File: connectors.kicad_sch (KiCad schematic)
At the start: 4 parts, among them J1 Conn_01x04_Pin, J2 Conn_01x04_Pin, J3 Conn_01x09_Pin, J4 Conn_02x03_Odd_Even

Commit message: Completed symbol-footprint associations
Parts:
- J1, J2: footprint (none) -> Connector_PinHeader_2.54mm:PinHeader_1x04_P2.54mm_Vertical
- J3: footprint (none) -> Connector_PinHeader_2.54mm:PinHeader_1x09_P2.54mm_Vertical
- J4: footprint (none) -> Connector_PinHeader_2.54mm:PinHeader_2x03_P2.54mm_Vertical
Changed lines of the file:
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@@
 			)
 		)
-		(property "Footprint" ""
+		(property "Footprint" "Connector_PinHeader_2.54mm:PinHeader_1x04_P2.54mm_Vertical"
 			(at 82.55 66.04 0)
 			(hide yes)
@@
 			)
 		)
-		(property "Footprint" ""
+		(property "Footprint" "Connector_PinHeader_2.54mm:PinHeader_1x04_P2.54mm_Vertical"
 			(at 60.96 66.04 0)
 			(hide yes)
@@
 			)
 		)
-		(property "Footprint" ""
+		(property "Footprint" "Connector_PinHeader_2.54mm:PinHeader_1x09_P2.54mm_Vertical"
 			(at 60.96 96.52 0)
 			(hide yes)
@@
 			)
 		)
-		(property "Footprint" ""
+		(property "Footprint" "Connector_PinHeader_2.54mm:PinHeader_2x03_P2.54mm_Vertical"
 			(at 83.82 90.17 0)
 			(hide yes)

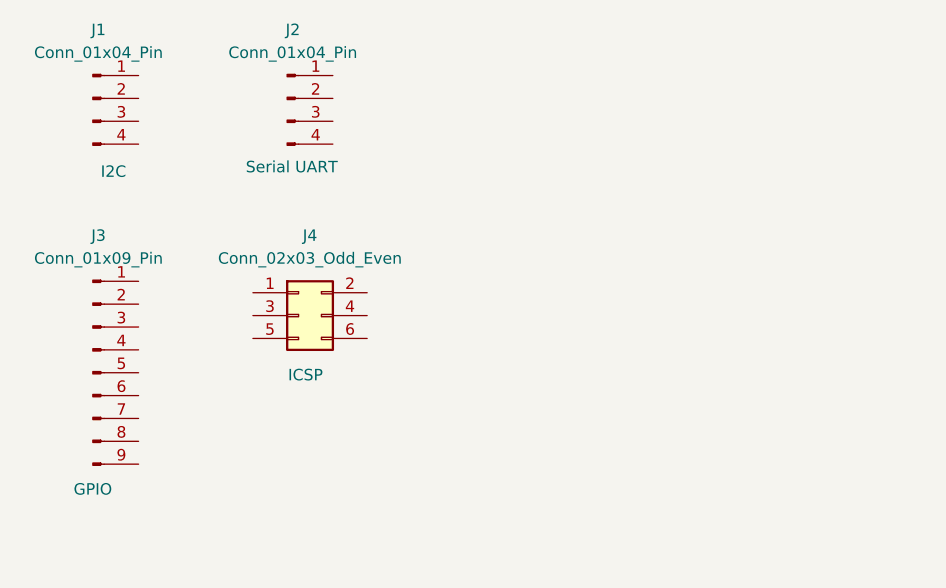
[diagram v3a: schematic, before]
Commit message: Completed wiring of the second sheet
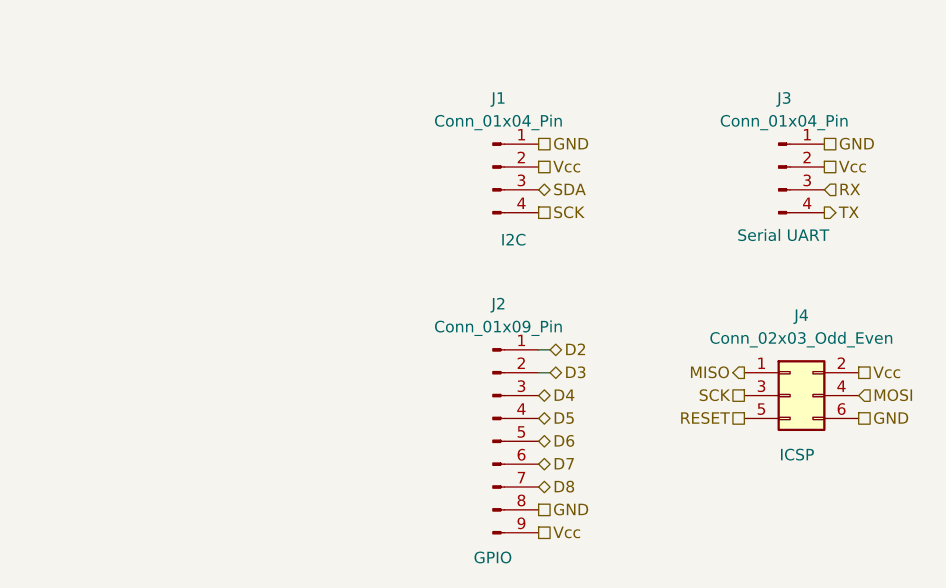
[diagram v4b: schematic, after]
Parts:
- renumbered J3 to J2, J2 to J3
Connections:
- net GND: now reaches J3.1 (Pin_1)
- net GND: now also J1.1 (Pin_1), J2.8 (Pin_8), J4.6 (Pin_6)
- net Vcc: now reaches J3.2 (Pin_2)
- net Vcc: now also J1.2 (Pin_2), J2.9 (Pin_9), J4.2 (Pin_2)
- net RX: now reaches J3.3 (Pin_3)
- net TX: now reaches J3.4 (Pin_4)
- net SDA: now reaches J1.3 (Pin_3)
- net SCK: now reaches J1.4 (Pin_4)
- net SCK: now also J4.3 (Pin_3)
- net D2: now reaches J2.1 (Pin_1)
- net D3: now reaches J2.2 (Pin_2)
- net D4: now reaches J2.3 (Pin_3)
- net D5: now reaches J2.4 (Pin_4)
- net D6: now reaches J2.5 (Pin_5)
- net D7: now reaches J2.6 (Pin_6)
- net D8: now reaches J2.7 (Pin_7)
- net MISO: now reaches J4.1 (Pin_1)
- net MOSI: now reaches J4.4 (Pin_4)
- net RESET: now reaches J4.5 (Pin_5)
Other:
- moved on the sheet: J1, J2, J3, J4
